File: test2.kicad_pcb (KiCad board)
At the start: 2 copper layers, 30.5 x 33 mm, 1 part

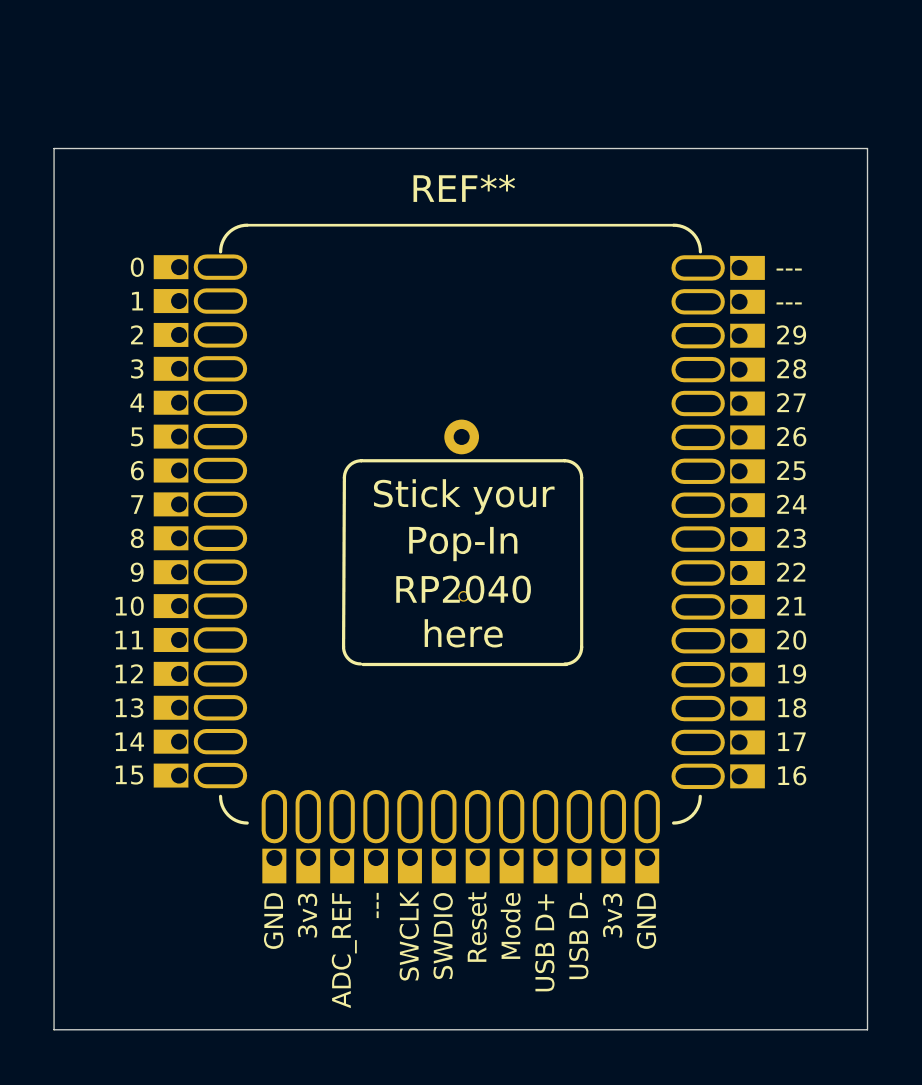
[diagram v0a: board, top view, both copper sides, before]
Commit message: Seriously messin' with 3D
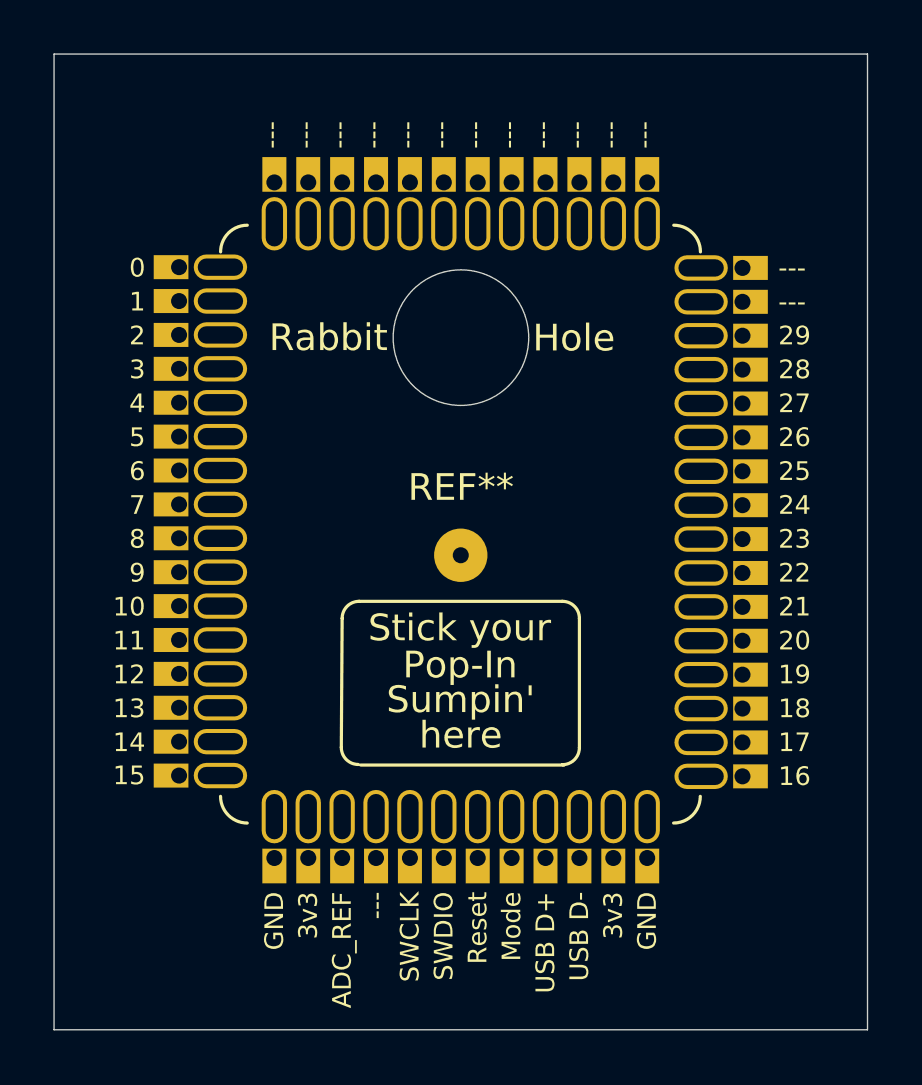
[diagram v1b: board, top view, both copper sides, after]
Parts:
- REF**: value NM-RP2040 (FlexyPin) -> NM-Generic-Module (FlexyPin); footprint Tinker RP2040:NM-RP2040 (FlexyPin) -> Tinker RP2040:NM-Generic-Module (FlexyPin)
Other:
- board size 30.5 x 33 mm -> 30.5 x 36.6 mm
- board text added: "Hole"
- board text added: "Rabbit"
